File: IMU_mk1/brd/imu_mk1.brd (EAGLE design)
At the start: 38.1 x 38.1 mm, 8 parts, among them U100 ATMEGA328PB

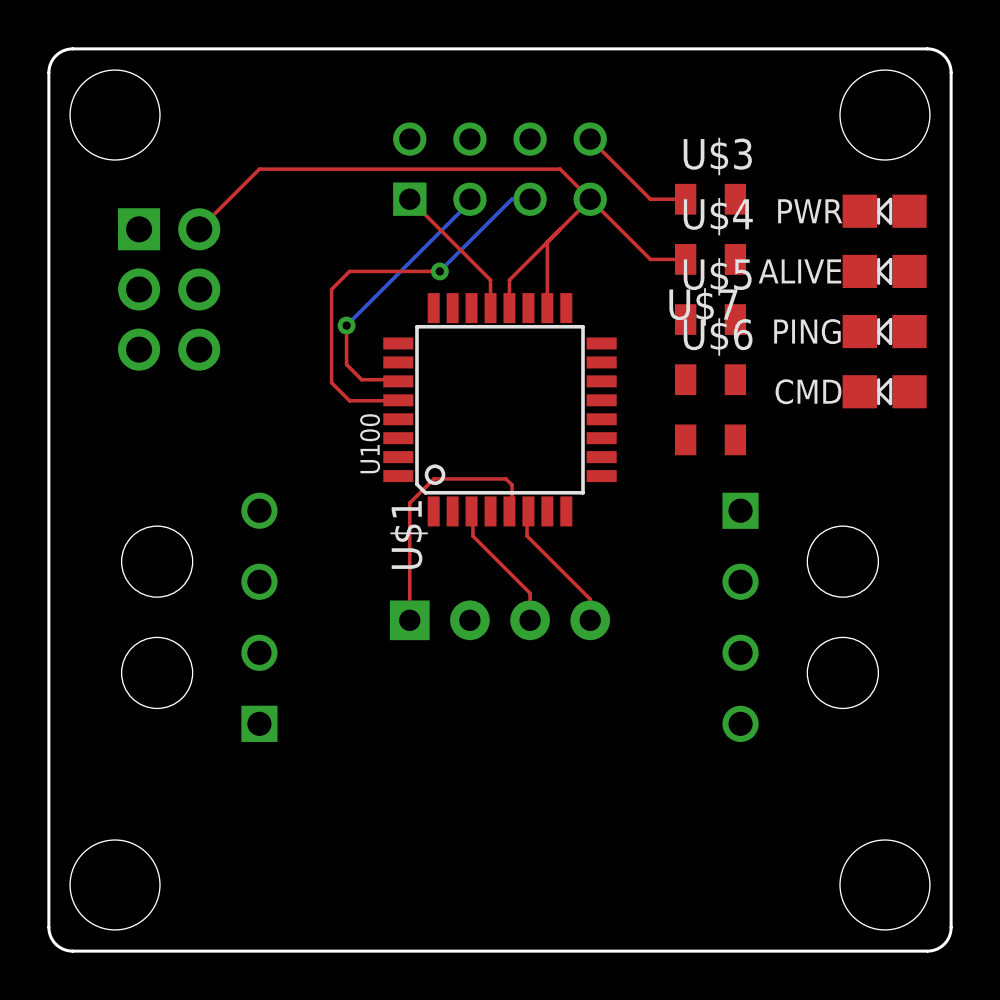
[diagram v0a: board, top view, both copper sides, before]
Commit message: IMU layout. GPS layout tweaks
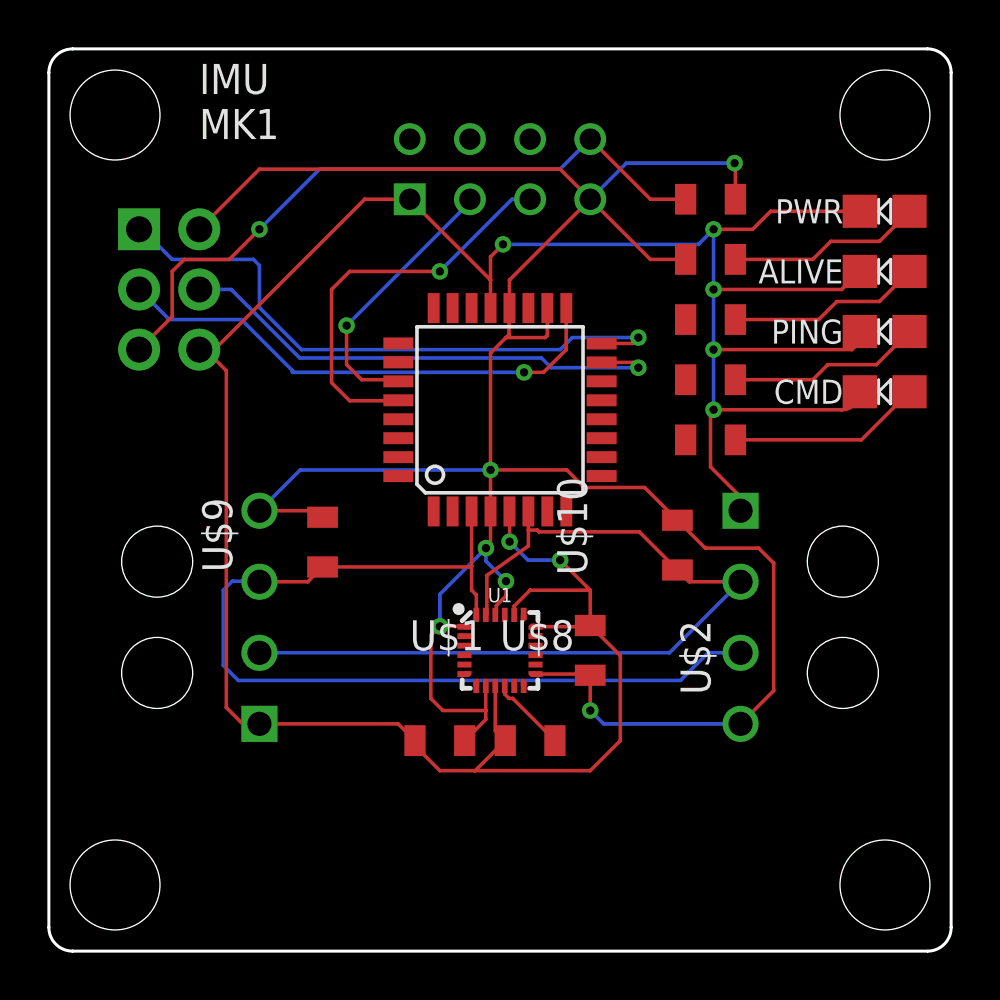
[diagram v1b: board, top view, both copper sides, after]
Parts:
- added U$10, U$2, U$8, U$9: (no value), 000_CustomPartsMaster:0805_STACKPOLERESISTOR
- added U1: 9DoF IMU, SparkFun-Sensors:QFN24-3X3
- IMU: value SENSOR_MODULE_MK1 -> MK1
- U$1: value 4PIN-HEADER -> (none); device 000_CustomPartsMaster:4HEADER_10MIL -> 000_CustomPartsMaster:0805_STACKPOLERESISTOR
- moved U$1 5.68 mm to (16.5, 8.89), turned to 0 degrees
- renumbered IMU_MK2 to IMU
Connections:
- new net REGOUT: U$8.P$2, U1.10
- net 3P3V: now also IMU.3P3V@2, IMU.3P3V@3, U$10.P$2, U$2.P$2, U$9.P$2, U1.1, U1.13, U1.22, U1.8
- net GND: now also IMU.GND@2, IMU.GND@3, U$2.P$1, U$8.P$1, U1.18, U1.20, U1.9
- net SCK: now also U100.17
- net SCL1: now also IMU.DATA1@1, IMU.DATA1@2, U$10.P$1, U1.23; no longer U$1.P$4
- net SDA1: now also IMU.DATA0@1, IMU.DATA0@2, U$9.P$1, U1.24; no longer U$1.P$3
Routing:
- net GND: track 17.0 -> 123.9 mm, vias 0 -> 7
- net 3P3V: track 32.7 -> 112.4 mm, vias 0 -> 6
- net SDA1: track 5.62 -> 41.1 mm
- net SCL1: track 5.73 -> 36.7 mm
- net MISO: track 0.00 -> 26.1 mm, vias 0 -> 1
- net RESET: track 5.08 -> 28.9 mm, vias 0 -> 1
- net SCK: track 0.00 -> 22.2 mm, vias 0 -> 1
- net MOSI: track 0.00 -> 21.7 mm, vias 0 -> 1
- net N$4: track 0.00 -> 8.19 mm
- net N$3: track 0.00 -> 8.19 mm
- net N$2: track 0.00 -> 8.19 mm
- net N$1: track 0.00 -> 8.19 mm
- net REGOUT: track 0.00 -> 3.28 mm
